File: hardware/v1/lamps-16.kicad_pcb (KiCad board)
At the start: 2 copper layers, 198.1 x 25.4 mm, 17 parts, among them P10 CONN_02X05

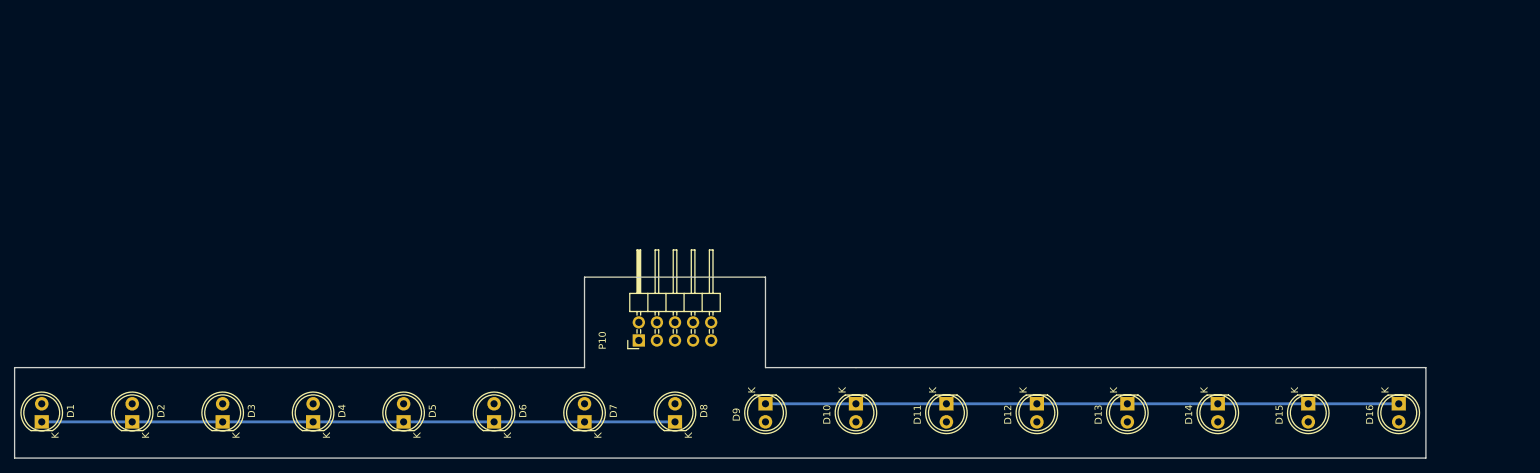
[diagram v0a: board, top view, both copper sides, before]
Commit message: Manually route lmaps-16 board
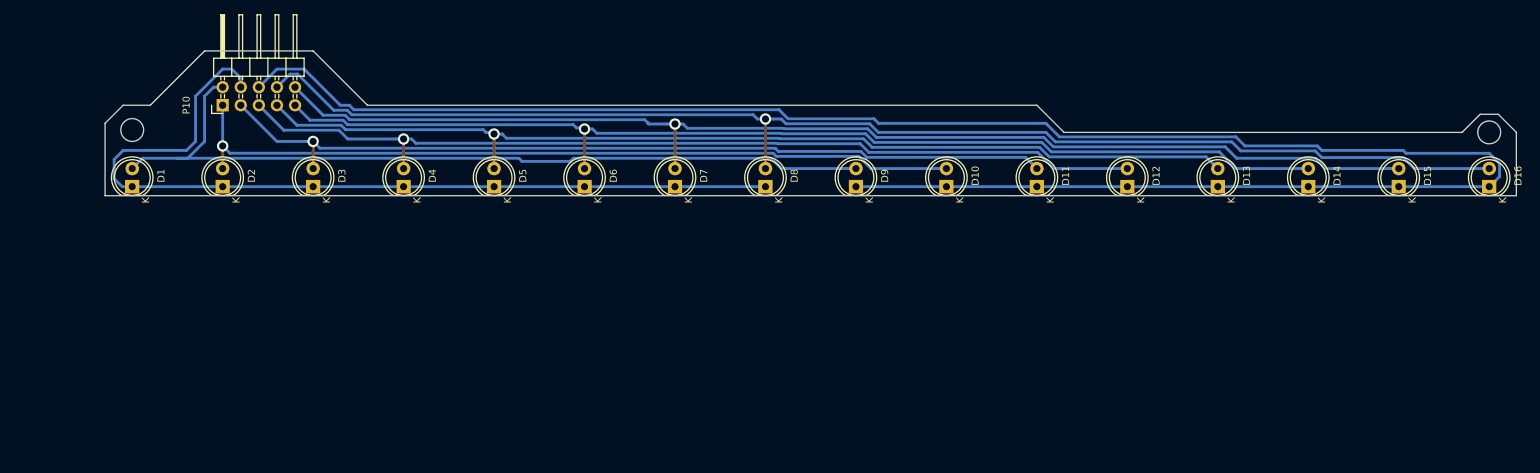
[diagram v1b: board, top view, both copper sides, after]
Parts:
- moved P10 67.1 mm to (50.8, 77.5)
- moved D1 35.4 mm to (38.1, 88.9)
- moved D3 35.4 mm to (63.5, 88.9)
- moved D4 35.4 mm to (76.2, 88.9)
- moved D5 35.4 mm to (88.9, 88.9)
- moved D7 35.4 mm to (114.3, 88.9)
- moved D8 35.4 mm to (127.0, 88.9)
- moved D2 35.4 mm to (50.8, 88.9)
- moved D6 35.4 mm to (101.6, 88.9)
- moved D10 33.0 mm to (152.4, 88.9), turned to 90 degrees
- moved D12 33.0 mm to (177.8, 88.9), turned to 90 degrees
- moved D15 33.0 mm to (215.9, 88.9), turned to 90 degrees
- moved D11 33.0 mm to (165.1, 88.9), turned to 90 degrees
- moved D13 33.0 mm to (190.5, 88.9), turned to 90 degrees
- moved D14 33.0 mm to (203.2, 88.9), turned to 90 degrees
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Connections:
- P10 pad 1: /SEG0 -> /SEG1
- P10 pad 10: /DIGITB -> /SEG6
- P10 pad 2: /SEG1 -> /SEG0
- P10 pad 4: /SEG3 -> /DIGITA
- P10 pad 5: /SEG4 -> /SEG3
- P10 pad 6: /SEG5 -> /DIGITB
- P10 pad 7: /SEG6 -> /SEG4
- P10 pad 9: /DIGITA -> /SEG5
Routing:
- net /DIGITB: track 88.9 -> 273.5 mm
- net /SEG7: track 0.00 -> 183.4 mm, vias 0 -> 1
- net /SEG6: track 0.00 -> 166.0 mm, vias 0 -> 1
- net /SEG5: track 0.00 -> 151.6 mm, vias 0 -> 1
- net /SEG4: track 0.00 -> 140.7 mm, vias 0 -> 1
- net /SEG3: track 0.00 -> 130.3 mm, vias 0 -> 1
- net /SEG2: track 0.00 -> 119.3 mm, vias 0 -> 1
- net /SEG0: track 0.00 -> 117.4 mm
- net /SEG1: track 0.00 -> 111.8 mm, vias 0 -> 1
- net /DIGITA: track 88.9 -> 123.2 mm
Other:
- board size 198.1 x 25.4 mm -> 198.1 x 20.3 mm
